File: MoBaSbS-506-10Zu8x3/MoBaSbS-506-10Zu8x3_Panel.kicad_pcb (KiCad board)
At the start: 2 copper layers, 63.8 x 64.8 mm, 21 parts, among them J1 Conn_02x05_Odd_Even, J10 1, J11 2, J12 3, J13 4

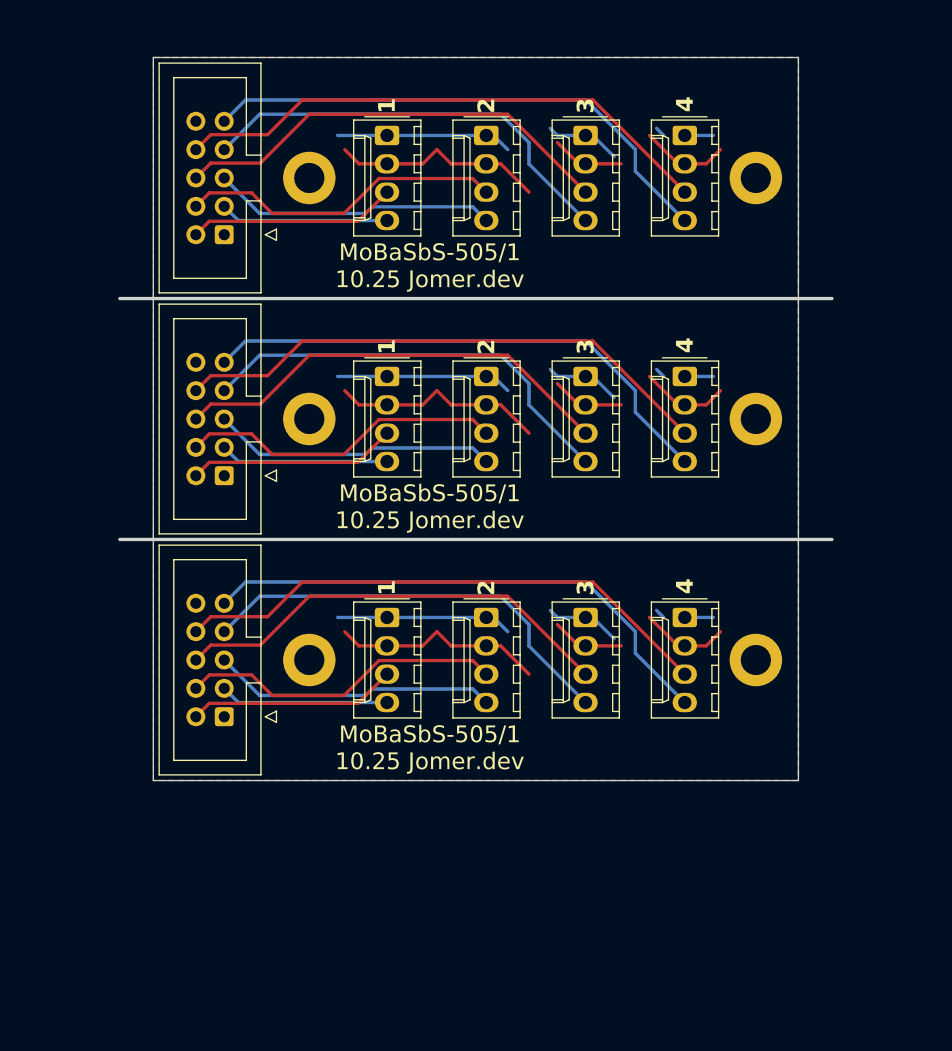
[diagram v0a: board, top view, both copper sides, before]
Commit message: Latest changes
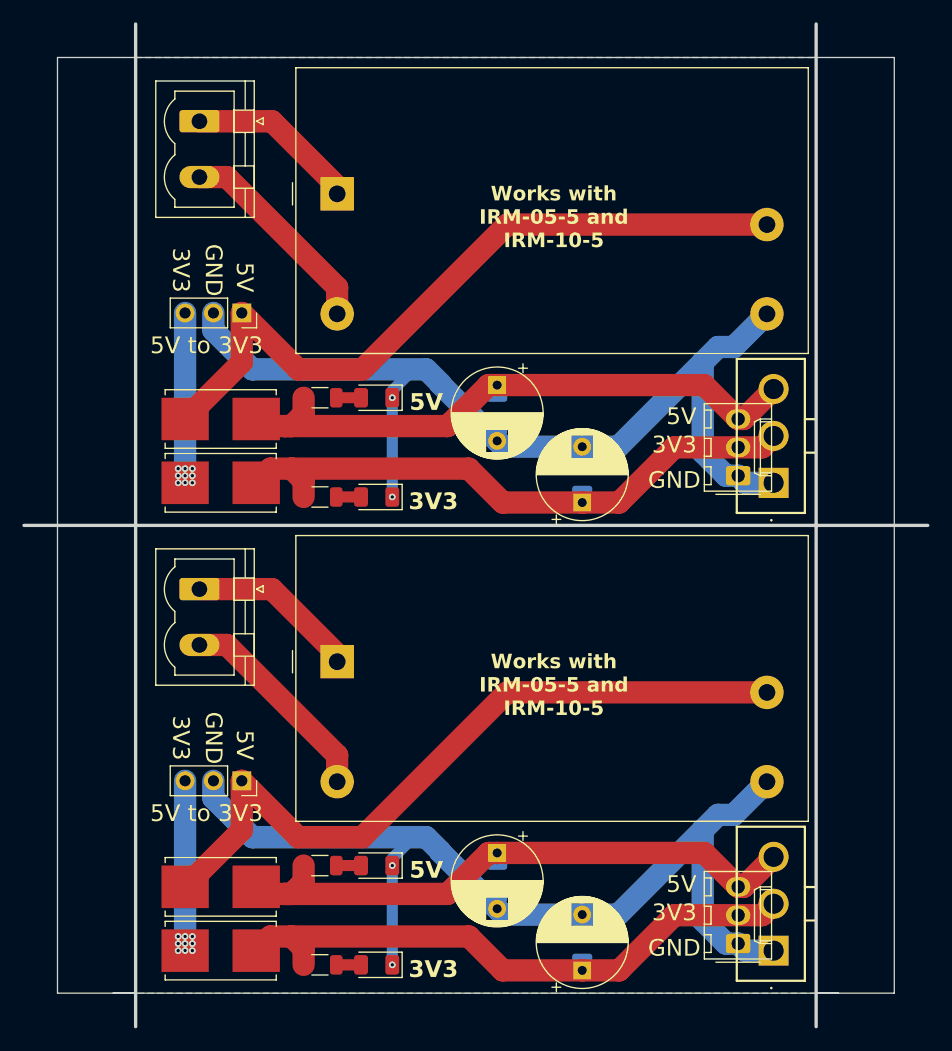
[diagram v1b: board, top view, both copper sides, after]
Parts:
- removed H1 (x3), H3 (x3): MountingHole_Pad, MountingHole:MountingHole_2.7mm_M2.5_DIN965_Pad
- removed the J1 at (126.0, 57.5)
- removed the J1 at (126.0, 35.9)
- removed the J1 at (126.0, 79.1)
- removed J10 (x3): 1, Connector_Molex:Molex_KK-254_AE-6410-04A_1x04_P2.54mm_Vertical
- removed J11 (x3): 2, Connector_Molex:Molex_KK-254_AE-6410-04A_1x04_P2.54mm_Vertical
- removed J12 (x3): 3, Connector_Molex:Molex_KK-254_AE-6410-04A_1x04_P2.54mm_Vertical
- removed J13 (x3): 4, Connector_Molex:Molex_KK-254_AE-6410-04A_1x04_P2.54mm_Vertical
- added C1: 470µF, Capacitor_THT:CP_Radial_D8.0mm_P5.00mm, F.Cu at (150.4, 91.3)
- added C1: 470µF, Capacitor_THT:CP_Radial_D8.0mm_P5.00mm, F.Cu at (150.4, 49.3)
- added C2: 470µF, Capacitor_THT:CP_Radial_D8.0mm_P5.00mm, F.Cu at (158.0, 59.9)
- added C2: 470µF, Capacitor_THT:CP_Radial_D8.0mm_P5.00mm, F.Cu at (158.0, 101.8)
- added C3: 100nF, Capacitor_SMD:C_1206_3216Metric, B.Cu at (150.4, 93.7)
- added C3: 100nF, Capacitor_SMD:C_1206_3216Metric, B.Cu at (150.4, 51.8)
- added C4: 100nF, Capacitor_SMD:C_1206_3216Metric, B.Cu at (158.0, 99.4)
- added C4: 100nF, Capacitor_SMD:C_1206_3216Metric, B.Cu at (158.0, 57.5)
- added D1: LED grün, LED_SMD:LED_1206_3216Metric, F.Cu at (139.6, 59.4)
- added D1: LED grün, LED_SMD:LED_1206_3216Metric, F.Cu at (139.6, 101.3)
- added D2: LED gelb, LED_SMD:LED_1206_3216Metric, F.Cu at (139.6, 92.4)
- added D2: LED gelb, LED_SMD:LED_1206_3216Metric, F.Cu at (139.6, 50.5)
- added F3: 1AT, Fuse:Fuseholder_Littelfuse_Nano2_154x, F.Cu at (125.6, 58.1)
- added F3: 1AT, Fuse:Fuseholder_Littelfuse_Nano2_154x, F.Cu at (125.6, 100.0)
- added F4: 2AT, Fuse:Fuseholder_Littelfuse_Nano2_154x, F.Cu at (125.6, 94.3)
- added F4: 2AT, Fuse:Fuseholder_Littelfuse_Nano2_154x, F.Cu at (125.6, 52.4)
- added J1: Conn_01x02, Connector_Phoenix_MSTB:PhoenixContact_MSTBVA_2,5_2-G_1x02_P5.00mm_Vertical, F.Cu at (123.7, 25.7)
- added J1: Conn_01x02, Connector_Phoenix_MSTB:PhoenixContact_MSTBVA_2,5_2-G_1x02_P5.00mm_Vertical, F.Cu at (123.7, 67.6)
- added J2: Conn_01x03, Connector_PinSocket_2.54mm:PinSocket_1x03_P2.54mm_Vertical, F.Cu at (127.5, 84.8)
- added J2: Conn_01x03, Connector_PinSocket_2.54mm:PinSocket_1x03_P2.54mm_Vertical, F.Cu at (127.5, 42.9)
- added J3: Power Out, Connector_Molex:Molex_KK-254_AE-6410-03A_1x03_P2.54mm_Vertical, F.Cu at (172.0, 57.5)
- added J3: Power Out, Connector_Molex:Molex_KK-254_AE-6410-03A_1x03_P2.54mm_Vertical, F.Cu at (172.0, 99.4)
- added J4: 43242-0005, Molex_MiniFitJr_1x3:Molex_MiniFitJr_1x3_PCB, F.Cu at (175.2, 58.1)
- added J4: 43242-0005, Molex_MiniFitJr_1x3:Molex_MiniFitJr_1x3_PCB, F.Cu at (175.2, 100.0)
- added PS1: IRM-10-5, Converter_ACDC:Converter_ACDC_MeanWell_IRM-10-xx_THT, F.Cu at (136.1, 74.1)
- added PS1: IRM-10-5, Converter_ACDC:Converter_ACDC_MeanWell_IRM-10-xx_THT, F.Cu at (136.1, 32.2)
- added R1: 1K0, Resistor_SMD:R_1206_3216Metric, F.Cu at (134.5, 59.4)
- added R1: 1K0, Resistor_SMD:R_1206_3216Metric, F.Cu at (134.5, 101.3)
- added R2: 2K2, Resistor_SMD:R_1206_3216Metric, F.Cu at (134.5, 50.5)
- added R2: 2K2, Resistor_SMD:R_1206_3216Metric, F.Cu at (134.5, 92.4)
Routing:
- net Board_1-GND: track 0.00 -> 88.3 mm, vias 0 -> 2
- net Board_0-GND: track 0.00 -> 88.3 mm, vias 0 -> 2
- net Board_0-/5V_PRE: track 0.00 -> 66.1 mm
- net Board_1-/5V_PRE: track 0.00 -> 66.1 mm
- net Board_1-/5V: track 0.00 -> 54.1 mm
- net Board_0-/5V: track 0.00 -> 54.1 mm
- net Board_1-/3V3: track 0.00 -> 53.6 mm
- net Board_0-/3V3: track 0.00 -> 53.6 mm
- net Board_2-/PIN_7: track 49.1 -> 0.00 mm
- net Board_0-/PIN_7: track 49.1 -> 0.00 mm
- net Board_1-/PIN_7: track 49.1 -> 0.00 mm
- net Board_2-/PIN_8: track 47.6 -> 0.00 mm
- net Board_1-/PIN_8: track 47.6 -> 0.00 mm
- net Board_0-/PIN_8: track 47.6 -> 0.00 mm
- net Board_1-/PIN_5: track 40.2 -> 0.00 mm
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- added copper zone on B.Cu, net Board_0-GND
- added copper zone on F.Cu, net Board_0-GND
- added copper zone on B.Cu, net Board_1-GND
- added copper zone on F.Cu, net Board_1-GND
- removed copper zone on F.Cu, net Board_0-/GND
- removed copper zone on B.Cu, net Board_0-/POWER
- removed copper zone on F.Cu, net Board_1-/GND
- removed copper zone on B.Cu, net Board_1-/POWER
- removed copper zone on F.Cu, net Board_2-/GND
- removed copper zone on B.Cu, net Board_2-/POWER
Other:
- board size 63.8 x 64.8 mm -> 81 x 89.8 mm
- board text added: "3V3"
- board text added: "5V"
- board text added: "5V to 3V3"
- board text added: "GND"
- board text added: "MA-507/1 10.25 Jomer.dev"
- board text added: "Works with IRM-05-5 and IRM-10-5"
- board text removed: "1"
- board text removed: "2"
- board text removed: "3"
- board text removed: "4"
- board text removed: "MoBaSbS-505/1 10.25 Jomer.dev"
